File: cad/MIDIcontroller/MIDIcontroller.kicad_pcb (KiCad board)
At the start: 2 copper layers, 49 parts, among them SW1 SW_SPST, SW2 SW_SPST, SW3 SW_SPST, SW4 SW_SPST, U0 74HC595

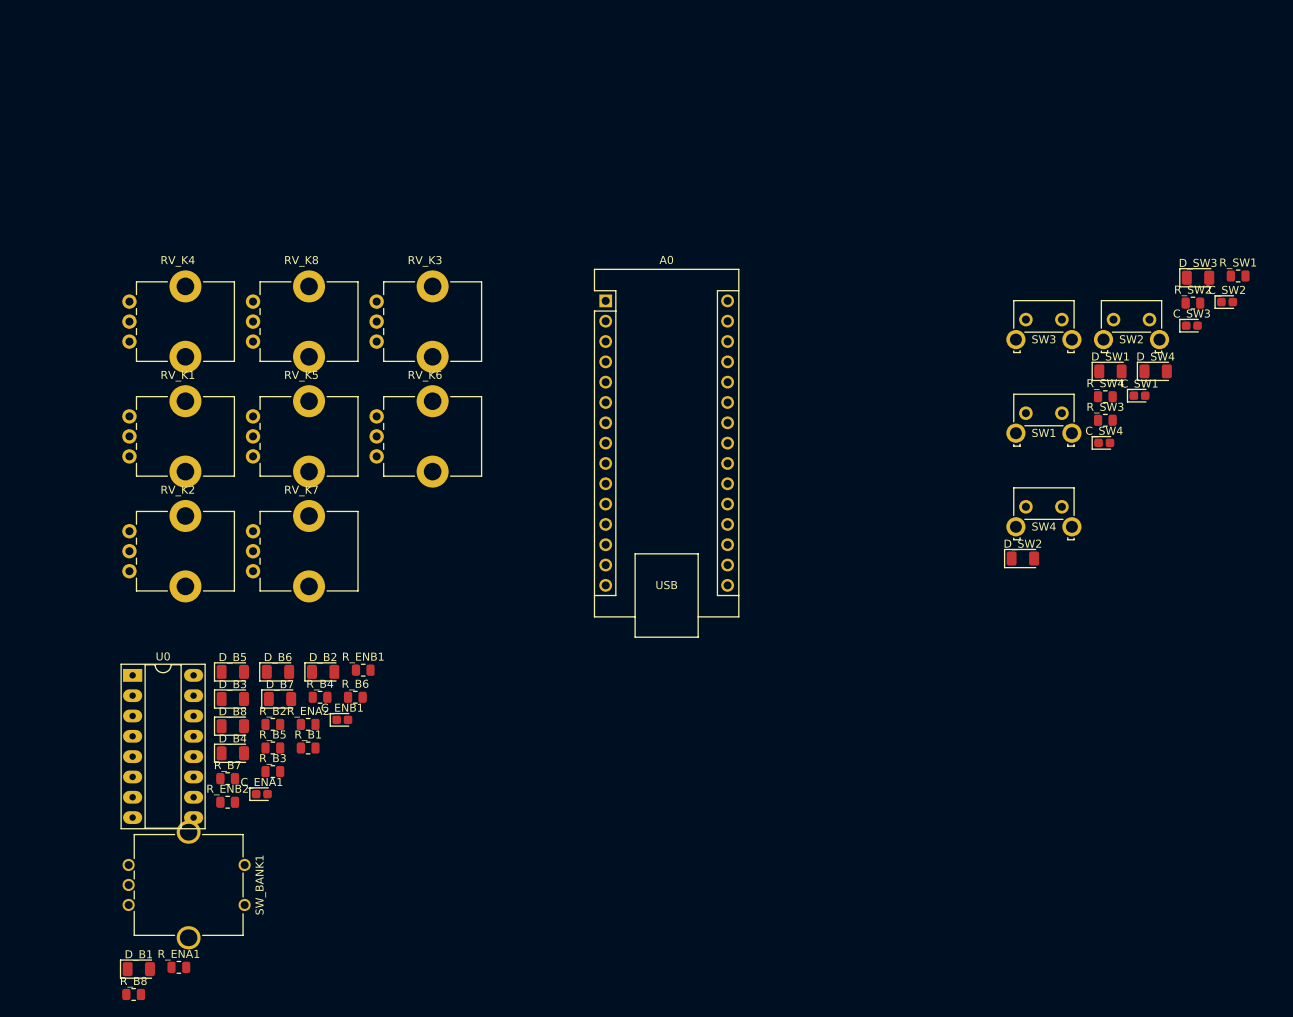
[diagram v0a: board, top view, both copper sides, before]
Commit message: Started routing
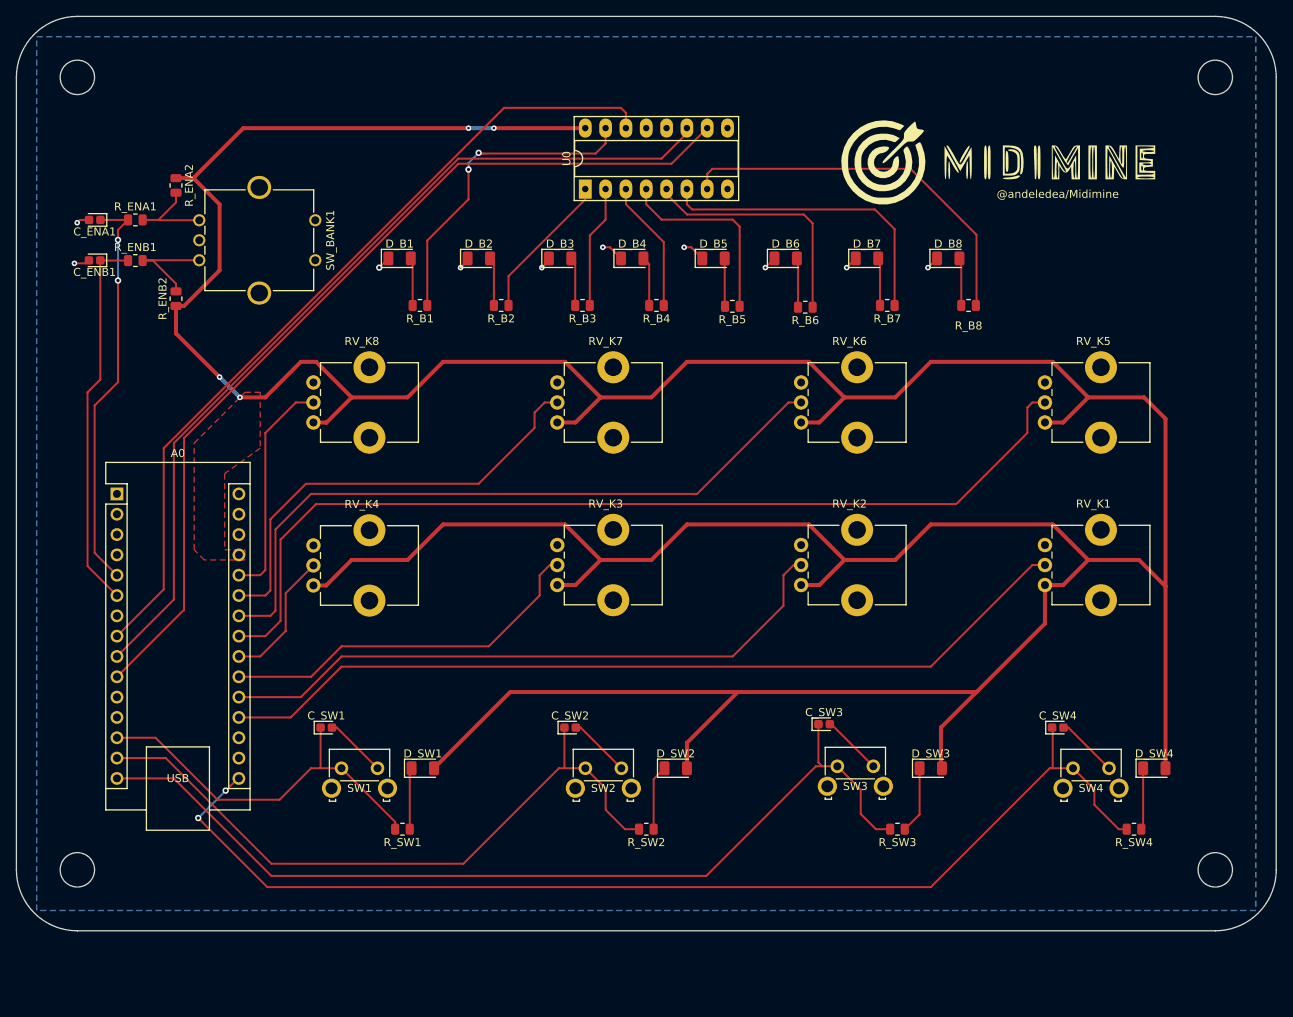
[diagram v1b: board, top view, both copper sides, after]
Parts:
- added G***: LOGO, LOGO, F.Cu at (189.2, 50.8)
- added H1: MountingHole, MountingHole:MountingHole_4.3mm_M4, F.Cu at (73.7, 40.6)
- added H2: MountingHole, MountingHole:MountingHole_4.3mm_M4, F.Cu at (215.9, 40.6)
- added H3: MountingHole, MountingHole:MountingHole_4.3mm_M4, F.Cu at (73.7, 139.7)
- added H4: MountingHole, MountingHole:MountingHole_4.3mm_M4, F.Cu at (215.9, 139.7)
- moved R_B8 135.3 mm to (185.1, 69.2), turned to 180 degrees
- moved R_SW1 125.3 mm to (114.3, 134.6), turned to 180 degrees
- moved RV_K1 115.6 mm to (194.6, 104.1)
- moved C_SW1 109.8 mm to (104.8, 121.9)
- moved D_B8 106.8 mm to (182.5, 63.3)
- moved R_B7 101.5 mm to (174.9, 69.2), turned to 180 degrees
- moved D_SW1 99.2 mm to (116.8, 127.0)
- moved RV_K5 99.1 mm to (194.6, 83.8)
- moved C_SW2 97.8 mm to (135.3, 121.9)
- moved SW1 96.4 mm to (106.7, 127.0)
- moved R_SW2 94.8 mm to (144.8, 134.6), turned to 180 degrees
- moved D_B1 94.6 mm to (113.9, 63.3)
- moved R_ENA1 93.6 mm to (80.9, 58.5)
- moved D_B7 91.7 mm to (172.4, 63.3)
- moved SW2 86.6 mm to (137.2, 127.0)
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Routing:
- net 5V: track 0.00 -> 542.8 mm, vias 0 -> 4
- net SW4: track 0.00 -> 142.3 mm, vias 0 -> 2
- net Knob5: track 0.00 -> 120.7 mm
- net SW3: track 0.00 -> 117.9 mm
- net STCP: track 0.00 -> 114.8 mm
- net SHCP: track 0.00 -> 110.4 mm
- net Knob1: track 0.00 -> 108.7 mm
- net DS: track 0.00 -> 103.5 mm
- net Knob6: track 0.00 -> 87.3 mm
- net SW2: track 0.00 -> 85.5 mm
- net Knob2: track 0.00 -> 79.4 mm
- net Knob7: track 0.00 -> 56.1 mm
- net Encoder_A: track 0.00 -> 50.8 mm, vias 0 -> 2
- net GND: track 0.00 -> 49.8 mm, vias 0 -> 10
- net SW1: track 0.00 -> 48.4 mm
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- added copper zone on F.Cu, net 5V
- added copper zone on B.Cu, net GND
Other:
- board outline added: 157.5 x 114.3 mm
- board text added: "@andeledea/Midimine"
